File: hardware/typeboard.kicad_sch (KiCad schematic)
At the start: 69 parts, among them J2 AXK6F20347YG

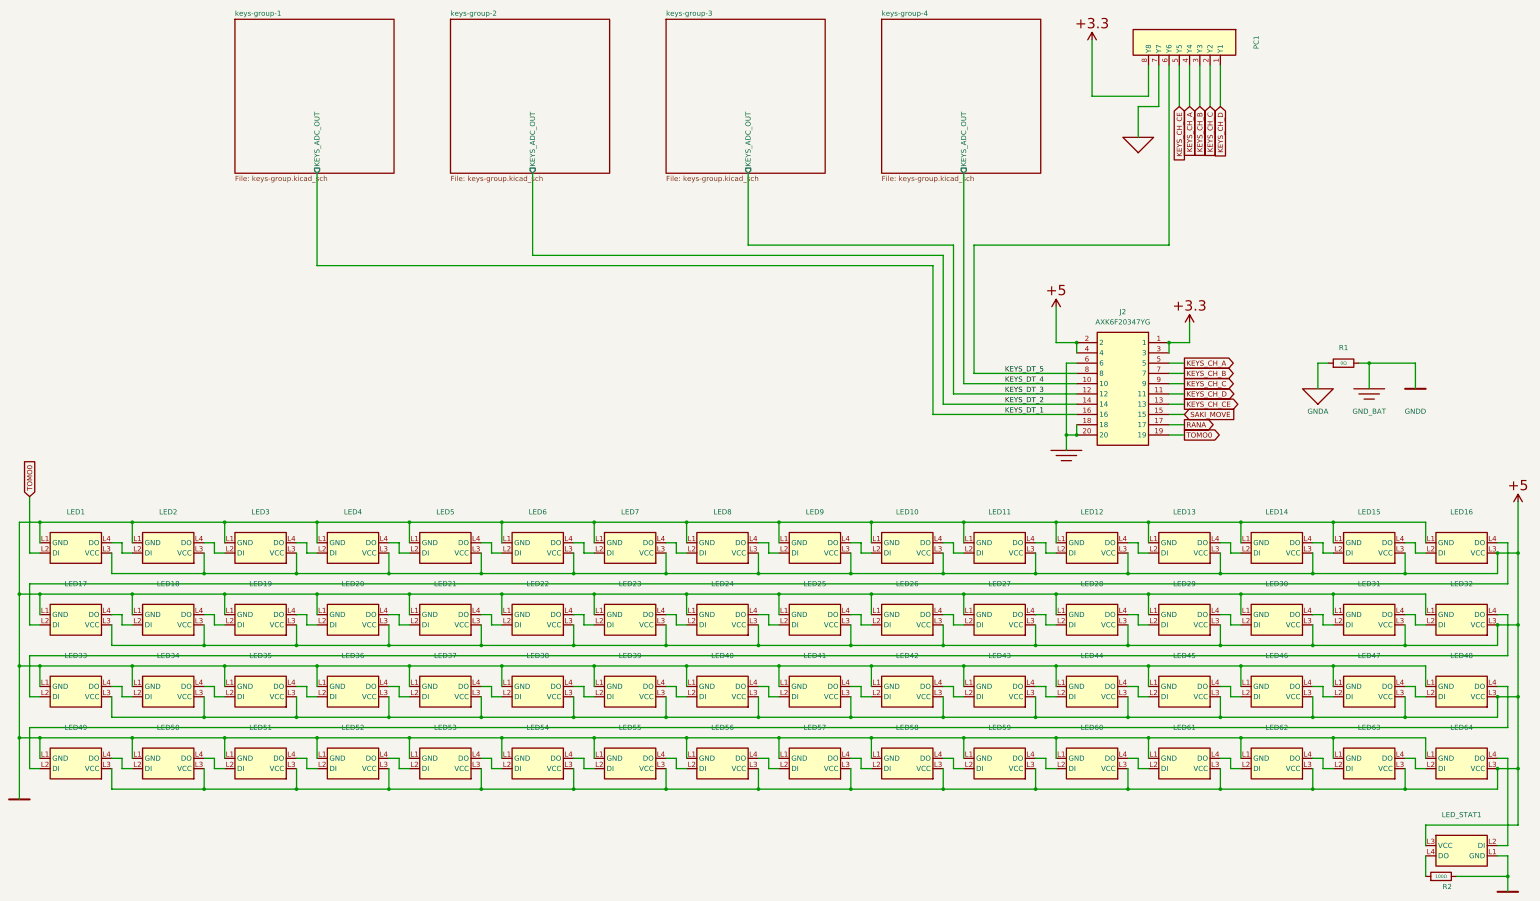
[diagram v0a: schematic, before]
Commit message: :sparkles: assembly all the part!
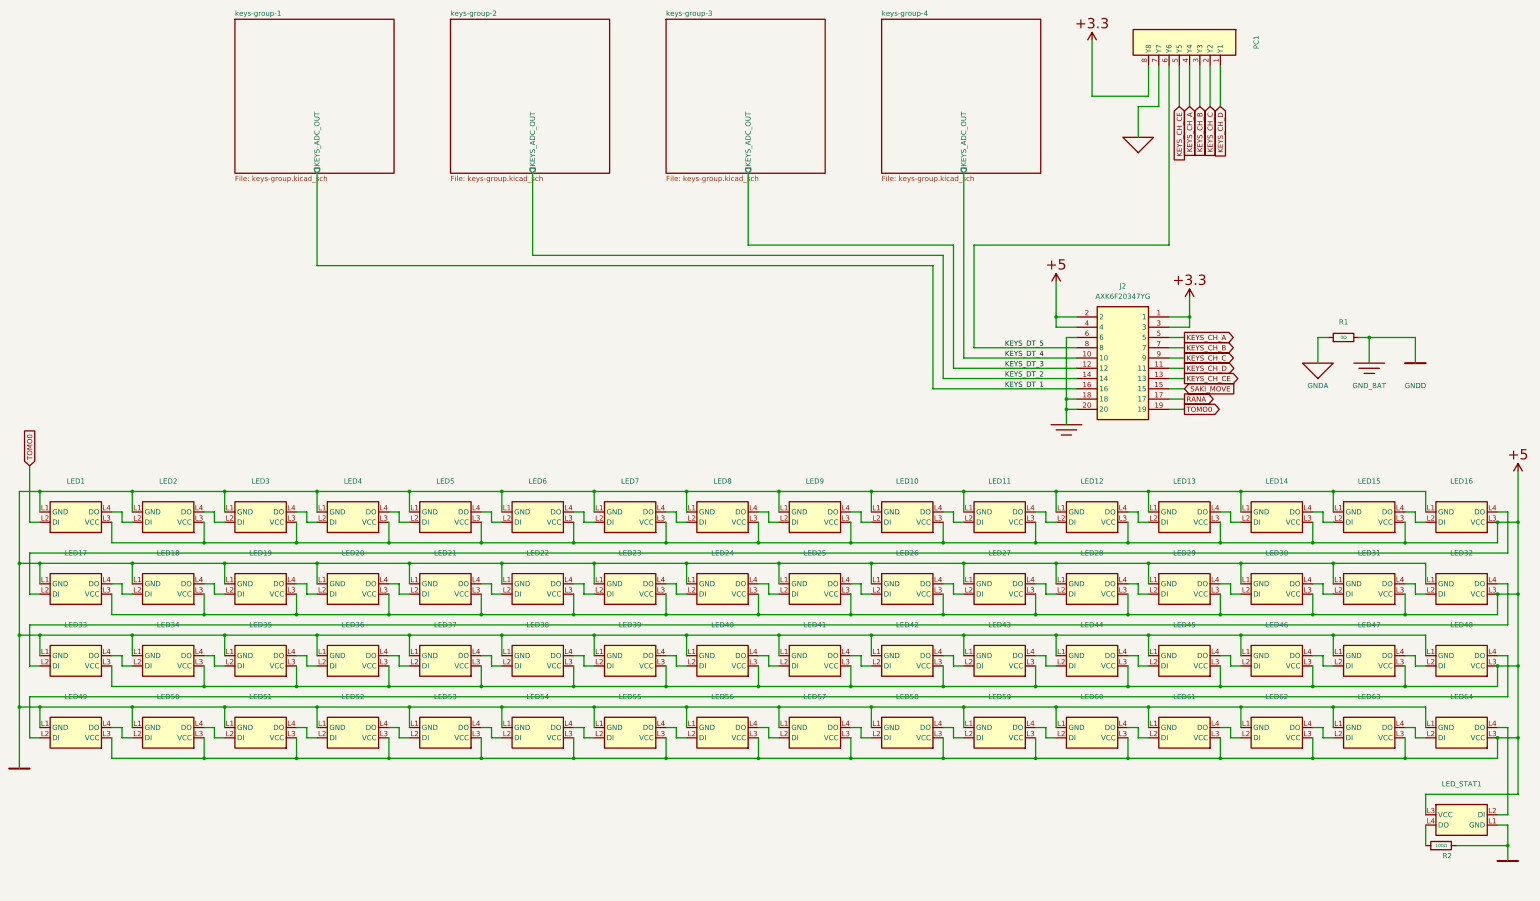
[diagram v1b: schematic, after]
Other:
- moved on the sheet: J2, LED1, LED10, LED11, LED12, LED13, LED14, LED15, LED16, LED17, LED18, LED19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
